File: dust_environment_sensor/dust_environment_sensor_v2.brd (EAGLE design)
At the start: 70.8 x 68.7 mm, 45 parts, among them IC2 ATMEGA644A, J1 3.6V Lithium C cell, J2 EXP, J3 XBEE_1-10SMT, J4 XBEE_11-20SMT, U1 LTP5901, U2 LIS3DH, U3 SI7005, U4 TSL2560, U5 AMN41121, U6 L3GD20, X2 32.768KHz

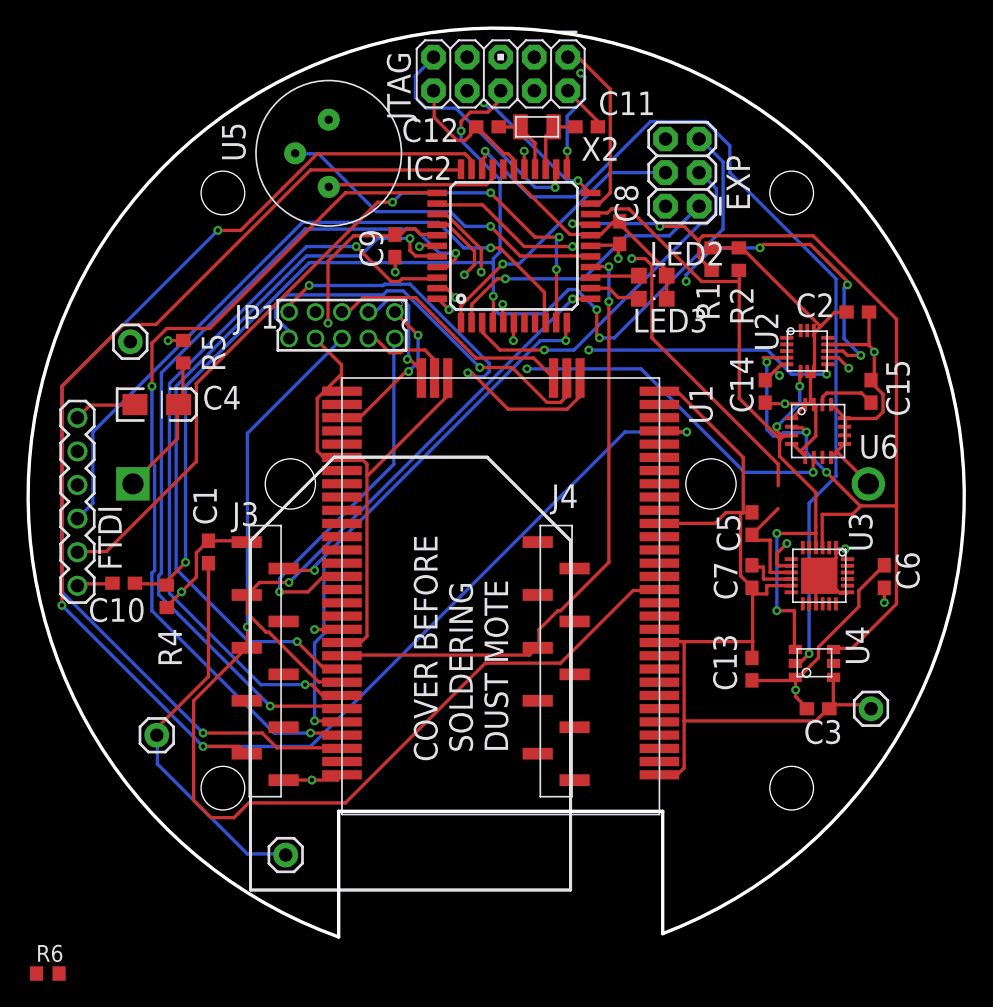
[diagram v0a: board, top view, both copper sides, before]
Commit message: changes for v2
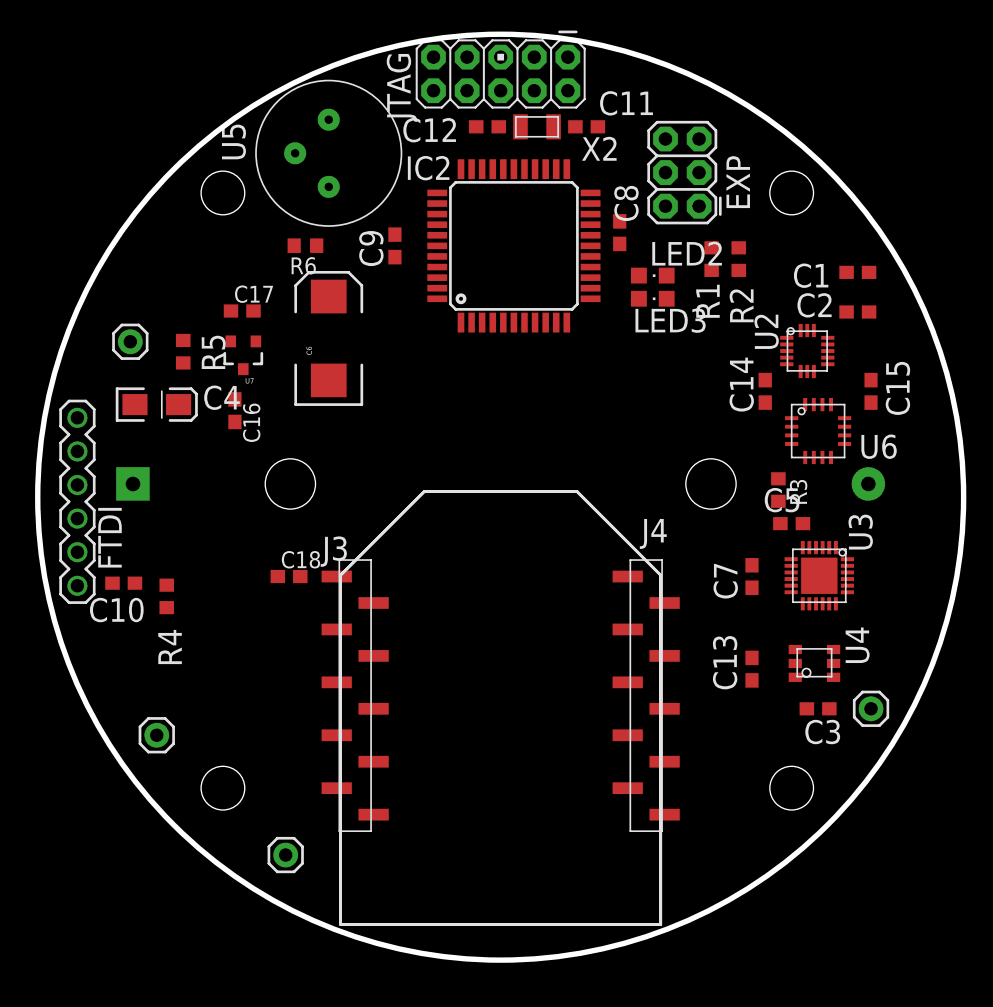
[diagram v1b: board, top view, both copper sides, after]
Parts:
- removed JP1: 87758-1016, con-molex:87758-1016
- removed U1: LTP5901, Cool_Electricity:LTP5901_MODULE
- added C16, C17: 1u, rcl:C0603
- added C18: 100n, rcl:C0603
- added R3: 15, resistor:R0603
- added U7: MCP1700-3.3V, Cool_Electricity:SOT23-3
- C6: value 100n -> 680u; device rcl:C0603 -> SparkFun-Capacitors:EIA7343
- R5: value 0R -> 0R DNP
- moved R6 58.4 mm to (20.2, 54.0), turned to 180 degrees
- moved C1 53.5 mm to (62.0, 52.0), turned to 0 degrees
- moved C6 45.7 mm to (22.0, 47.0), turned to 90 degrees
- moved J3 7.29 mm to (35.0, 20.0)
- moved J4 7.29 mm to (35.0, 20.0)
- moved C5 3.00 mm to (57.0, 33.0), turned to 0 degrees
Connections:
- removed net FLASH_P_ENN: JP1.2, U1.51
- removed net IPCS_MISO: JP1.5, U1.33
- removed net IPCS_MOSI: JP1.4, U1.35
- removed net IPCS_SCK: JP1.3, U1.36
- removed net IPCS_SSN: JP1.1, U1.39
- removed net MOTE_CLI_RX: JP1.10, U1.32
- removed net MOTE_CLI_TX: JP1.9, U1.31
- removed net MOTE_RADIO_INHIBIT: IC2.32, U1.64
- removed net MOTE_RX_CTSN: IC2.40, U1.58
- removed net MOTE_TIMEN: IC2.34, U1.63
- removed net MOTE_TX_RTSN: IC2.42, U1.60
- new net HUMID_VCC: IC2.34, R3.1
- new net MOTE_ASSOC: IC2.41, J4.15
- new net MOTE_STATUS: IC2.42, J4.13
- new net N$11: C5.1, R3.2, U3.9
- net GND: now also C16.2, C17.2, C18.1, C6.C, U7.1; no longer C6.2, JP1.8, U1.1, U1.11, U1.20, U1.30, U1.34, U1.37, U1.42, U1.56, U1.66
- net MOTE_API_RX: no longer U1.59
- net MOTE_API_TX: no longer U1.62
- net MOTE_RESETN: now also IC2.33; no longer JP1.6, U1.15
- net MOTE_RX_RTSN: no longer U1.57
- net MOTE_SLEEPN: now also IC2.32; no longer IC2.33, U1.27
- net MOTE_TX_CTSN: now also IC2.40, J4.12; no longer IC2.41, U1.61
- net VBATT: now also C16.1, J2.2, JP8.3, U7.3
- net VCC: now also C17.1, C18.2, C6.A, U7.2; no longer C5.1, C6.1, J2.2, JP1.7, U1.55, U3.9
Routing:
- net GND: track 231.6 -> 0.00 mm, vias 10 -> 0
- net MOTE_SLEEPN: track 120.7 -> 0.00 mm, vias 3 -> 0
- net VCC: track 92.3 -> 0.00 mm, vias 9 -> 0
- net I2C_SCL: track 87.1 -> 0.00 mm, vias 5 -> 0
- net MOTE_RESETN: track 82.5 -> 0.00 mm, vias 1 -> 0
- net MOTE_RADIO_INHIBIT: track 80.8 -> 0.00 mm, vias 2 -> 0
- net LIGHT_INT: track 68.4 -> 0.00 mm, vias 2 -> 0
- net RST: track 66.3 -> 0.00 mm, vias 3 -> 0
- net MOTE_TIMEN: track 64.9 -> 0.00 mm, vias 2 -> 0
- net MOTE_TX_CTSN: track 63.9 -> 0.00 mm, vias 2 -> 0
- net ATMEGA_TO_FTDI: track 59.1 -> 0.00 mm, vias 4 -> 0
- net MOTE_TX_RTSN: track 57.9 -> 0.00 mm, vias 2 -> 0
- net I2C_SDA: track 57.1 -> 0.00 mm, vias 4 -> 0
- net MOTE_RX_CTSN: track 55.0 -> 0.00 mm, vias 2 -> 0
- net FTDI_TO_ATMEGA: track 52.3 -> 0.00 mm, vias 1 -> 0
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- removed copper zone on layer 15, net GND
- removed copper zone on layer 2, net VCC
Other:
- board size 70.8 x 68.7 mm -> 70 x 70 mm
- board text added: "Environmental Sensor PCB Kevin Weekly"
- board text removed: "COVER BEFORE SOLDERING DUST MOTE"
- board text removed: "Dust Sensor PCB Kevin Weekly"

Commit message: Test golden version of ES2
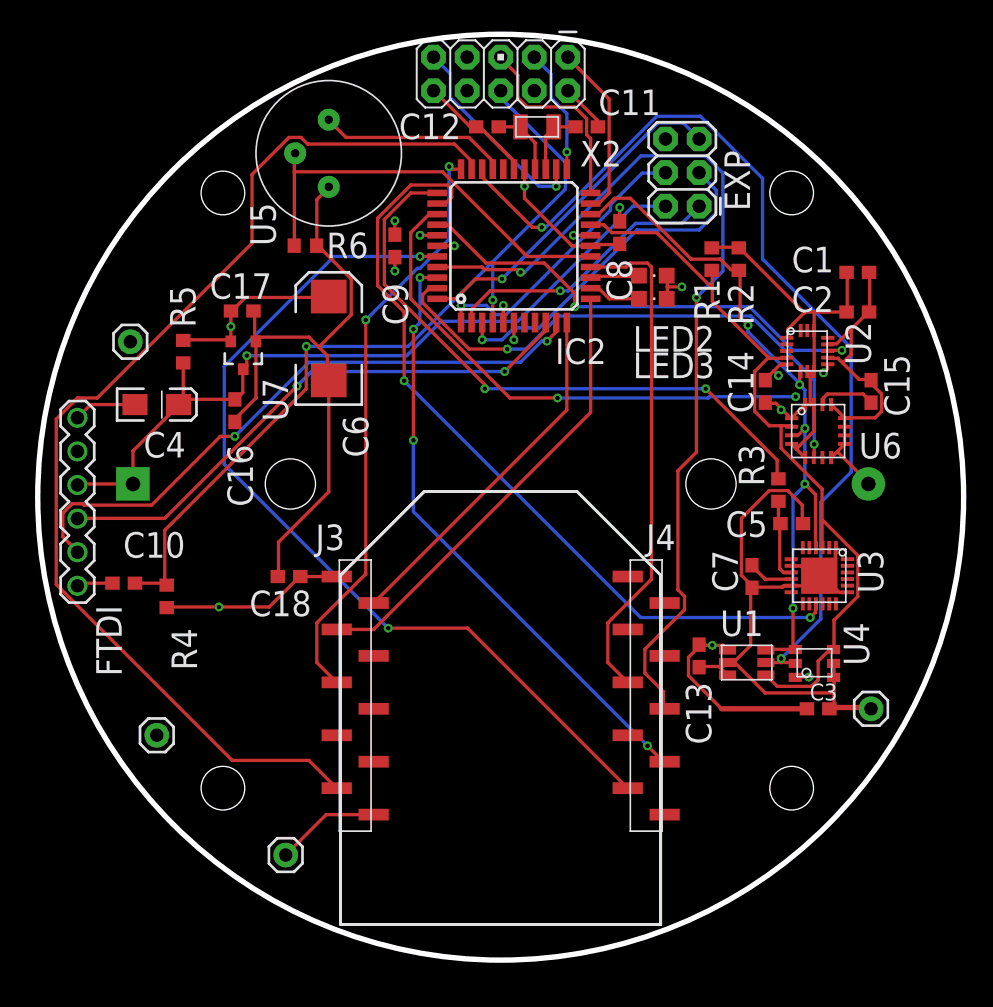
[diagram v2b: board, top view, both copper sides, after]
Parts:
- added U1: TSL2560T, Cool_Electricity:T_TAOS
- U4: value TSL2560 -> TSL2560CL
- moved C13 4.12 mm to (50.0, 23.0), turned to 270 degrees
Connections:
- net GND: now also U1.2, U1.3
- net I2C_SCL: now also U1.4
- net I2C_SDA: now also U1.6
- net LIGHT_INT: now also U1.5
- net VCC: now also U1.1
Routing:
- net GND: track 0.00 -> 165.4 mm, vias 0 -> 7
- net VCC: track 0.00 -> 93.8 mm, vias 0 -> 9
- net MOTE_SLEEPN: track 0.00 -> 84.7 mm
- net LIGHT_INT: track 0.00 -> 72.6 mm, vias 0 -> 2
- net MOTE_ASSOC: track 0.00 -> 70.0 mm, vias 0 -> 2
- net MOTE_TX_CTSN: track 0.00 -> 67.6 mm, vias 0 -> 2
- net RST: track 0.00 -> 63.5 mm, vias 0 -> 2
- net HUMID_CS: track 0.00 -> 61.1 mm, vias 0 -> 2
- net VBATT: track 0.00 -> 59.5 mm, vias 0 -> 1
- net I2C_SCL: track 0.00 -> 58.4 mm
- net I2C_SDA: track 0.00 -> 54.9 mm, vias 0 -> 5
- net ATMEGA_TO_FTDI: track 0.00 -> 47.2 mm, vias 0 -> 2
- net HUMID_VCC: track 0.00 -> 46.6 mm, vias 0 -> 2
- net MOTE_STATUS: track 0.00 -> 46.0 mm, vias 0 -> 4
- net MOTE_RESETN: track 0.00 -> 44.9 mm, vias 0 -> 2
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- added copper zone on layer 15, net GND
- added copper zone on layer 2, net VCC
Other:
- board text removed: "JTAG"
